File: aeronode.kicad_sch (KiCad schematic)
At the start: 8 parts

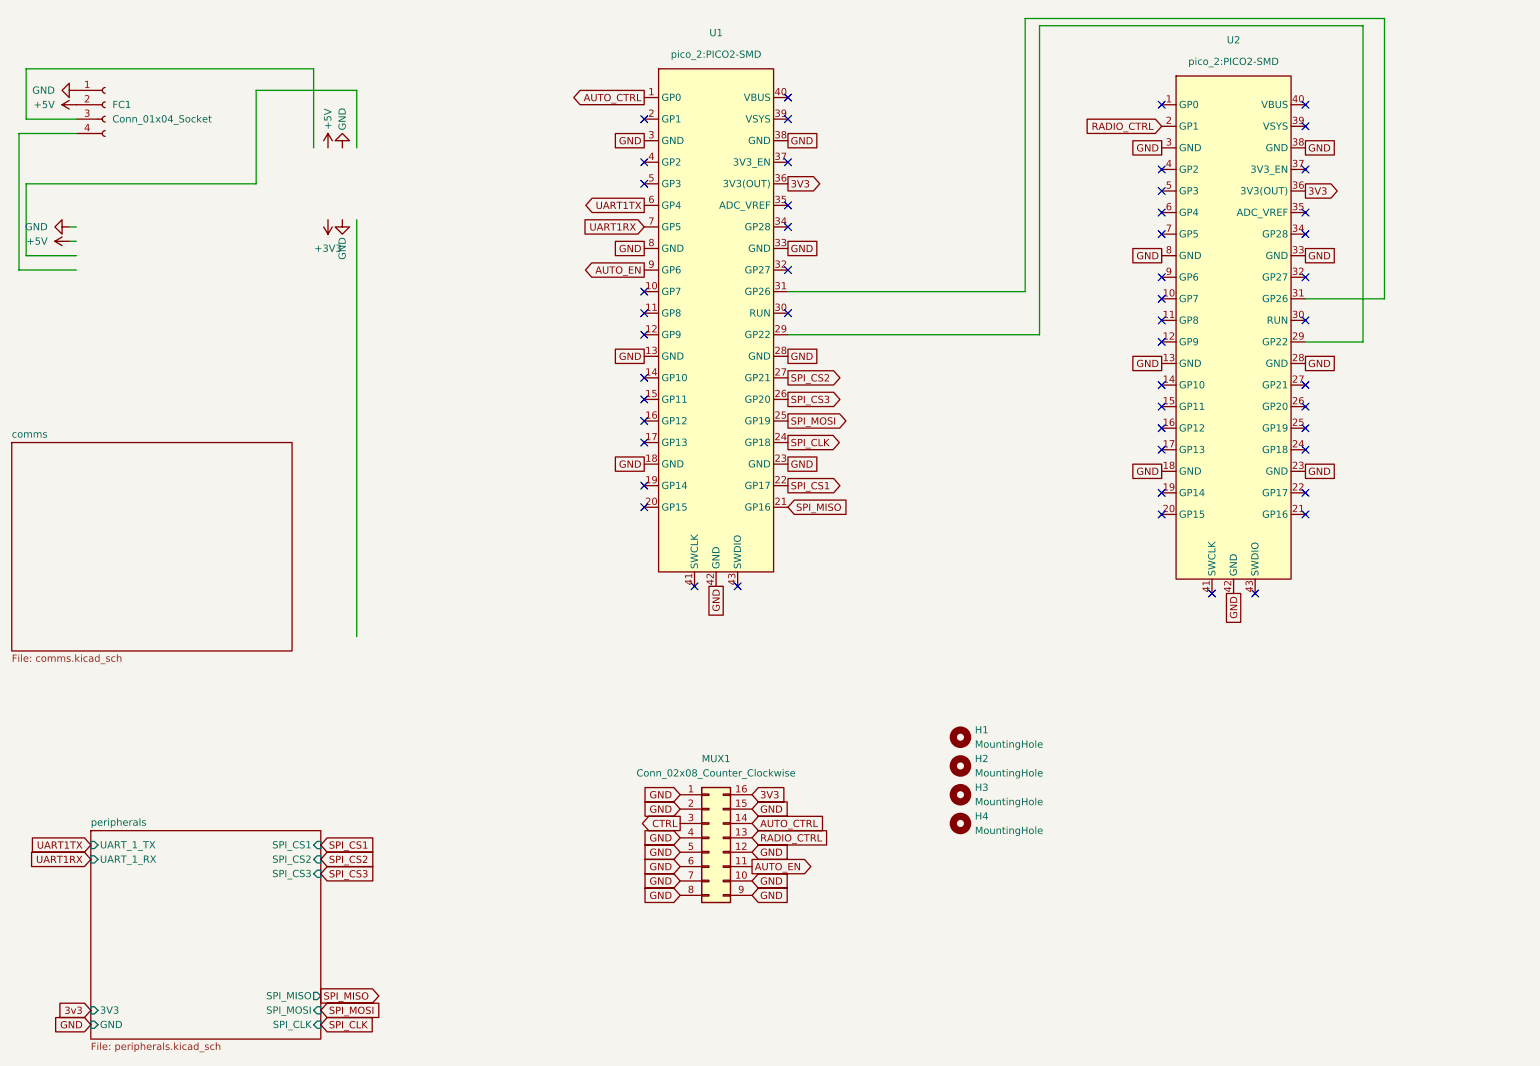
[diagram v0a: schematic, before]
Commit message: v0.1
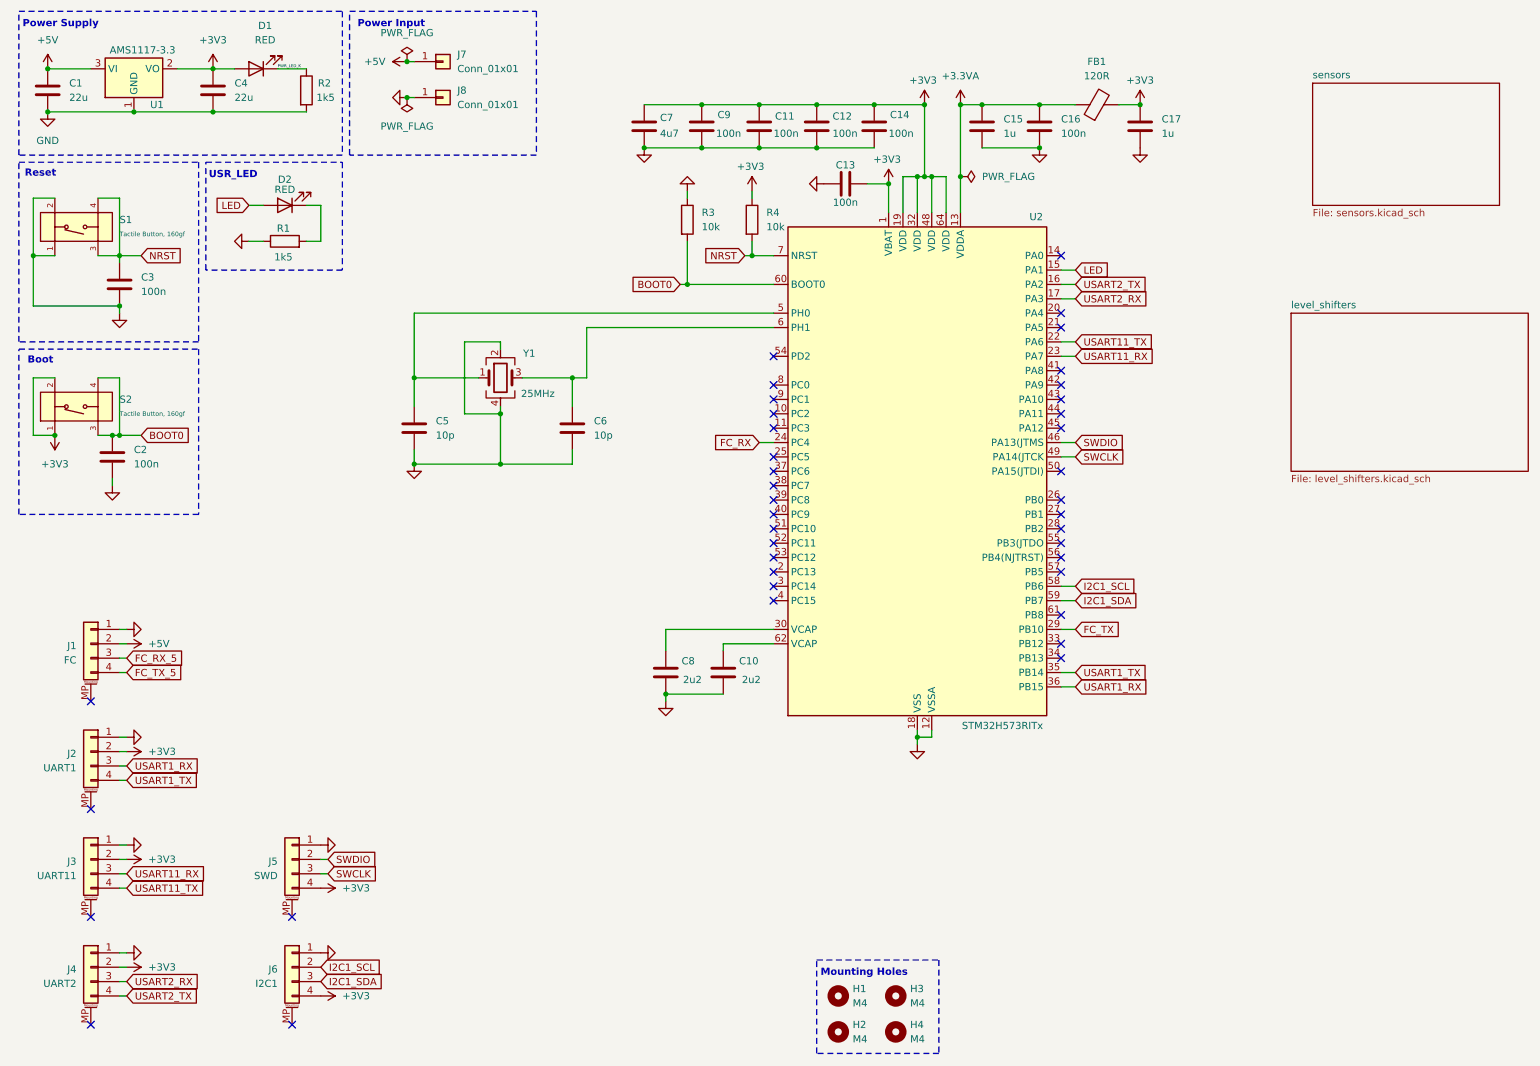
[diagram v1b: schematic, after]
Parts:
- removed FC1: Conn_01x04_Socket, Connector_PinSocket_2.54mm:PinSocket_1x04_P2.54mm_Vertical, symbol Connector:Conn_01x04_Socket
- removed MUX1: Conn_02x08_Counter_Clockwise, Connector_PinHeader_2.54mm:PinHeader_2x8_2.54mm_7.62mm, symbol Connector_Generic:Conn_02x08_Counter_Clockwise
- removed U1, U2: ~, pico_2:PICO2-SMD, symbol pico_2:PICO2-SMD
- added C1, C4: 22u, Capacitor_SMD:C_0805_2012Metric, symbol Device:C
- added C10, C8: 2u2, Capacitor_SMD:C_0402_1005Metric, symbol Device:C
- added C11, C12, C13, C14, C16, C2, C3, C9: 100n, Capacitor_SMD:C_0402_1005Metric, symbol Device:C
- added C15, C17: 1u, Capacitor_SMD:C_0402_1005Metric, symbol Device:C
- added C5, C6: 10p, Capacitor_SMD:C_0402_1005Metric, symbol Device:C
- added C7: 4u7, Capacitor_SMD:C_0603_1608Metric, symbol Device:C
- added D1, D2: RED, LED_SMD:LED_0603_1608Metric, symbol Device:LED
- added FB1: 120R, Inductor_SMD:L_0603_1608Metric, symbol Device:FerriteBead
- added J1: FC, Connector_JST:JST_GH_SM04B-GHS-TB_1x04-1MP_P1.25mm_Horizontal, symbol Connector_Generic_MountingPin:Conn_01x04_MountingPin
- added J2: UART1, Connector_JST:JST_GH_SM04B-GHS-TB_1x04-1MP_P1.25mm_Horizontal, symbol Connector_Generic_MountingPin:Conn_01x04_MountingPin
- added J3: UART11, Connector_JST:JST_GH_SM04B-GHS-TB_1x04-1MP_P1.25mm_Horizontal, symbol Connector_Generic_MountingPin:Conn_01x04_MountingPin
- added J4: UART2, Connector_JST:JST_GH_SM04B-GHS-TB_1x04-1MP_P1.25mm_Horizontal, symbol Connector_Generic_MountingPin:Conn_01x04_MountingPin
- added J5: SWD, Connector_JST:JST_GH_SM04B-GHS-TB_1x04-1MP_P1.25mm_Horizontal, symbol Connector_Generic_MountingPin:Conn_01x04_MountingPin
- added J6: I2C1, Connector_JST:JST_GH_SM04B-GHS-TB_1x04-1MP_P1.25mm_Horizontal, symbol Connector_Generic_MountingPin:Conn_01x04_MountingPin
- added J7, J8: Conn_01x01, Connector_Wire:SolderWirePad_1x01_SMD_2x4mm, symbol Connector_Generic:Conn_01x01
- added R1, R2: 1k5, Resistor_SMD:R_0402_1005Metric, symbol Device:R
- added R3, R4: 10k, Resistor_SMD:R_0402_1005Metric, symbol Device:R
- added S1, S2: Tactile Button, 160gf, PCM_JLCPCB:SW-SMD_4P-L5.1-W5.1-P3.70-LS6.5-TL-2, symbol PCM_JLCPCB-Connectors_Buttons:Tactile Button, 160gf, 12V, 50mA, 5.1mm
- added U1: AMS1117-3.3, Package_TO_SOT_SMD:SOT-223-3_TabPin2, symbol Regulator_Linear:AMS1117-3.3
- added U2: STM32H573RITx, Package_QFP:LQFP-64_10x10mm_P0.5mm, symbol MCU_ST_STM32H5:STM32H573RITx
- added Y1: 25MHz, Crystal:Crystal_SMD_3225-4Pin_3.2x2.5mm, symbol Device:Crystal_GND24
- H1, H2, H3, H4: value MountingHole -> M4; footprint (none) -> MountingHole:MountingHole_4.3mm_M4
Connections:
- net +3V3: now also C11.1, C12.1, C13.2, C14.1, C17.2, C4.1, C7.1, C9.1, D1.2 (A), FB1.2, J2.2 (Pin_2), J3.2 (Pin_2), J4.2 (Pin_2), J5.4 (Pin_4), J6.4 (Pin_4), R4.1, S2.1 (A), S2.2 (B), U1.2 (VO), U2.1 (VBAT), U2.19 (VDD), U2.32 (VDD), U2.48 (VDD), U2.64 (VDD)
- net +5V: now also C1.1, J1.2 (Pin_2), J7.1 (Pin_1), U1.3 (VI)
- net GND: now also C1.2, C10.2, C11.2, C12.2, C13.1, C14.2, C15.1, C16.1, C17.1, C2.2, C3.2, C4.2, C5.2, C6.2, C7.2, C8.2, C9.2, J1.1 (Pin_1), J2.1 (Pin_1), J3.1 (Pin_1), J4.1 (Pin_1), J5.1 (Pin_1), J6.1 (Pin_1), J8.1 (Pin_1), R1.1, R2.2, R3.1, S1.1 (A), S1.2 (B), U1.1 (GND), U2.12 (VSSA), U2.18 (VSS), U2.31 (VSS), U2.47 (VSS), U2.63 (VSS), Y1.2, Y1.4
- new net: C8.1, U2.30 (VCAP)
- new net: C5.1, U2.5 (PH0), Y1.1
- new net: C6.1, U2.6 (PH1), Y1.3
- new net: C10.1, U2.62 (VCAP)
- new net: D2.1 (K), R1.2
- new net +3.3VA: C15.2, C16.2, FB1.1, U2.13 (VDDA)
- new net BOOT0: C2.1, R3.2, S2.3 (C), S2.4 (D), U2.60 (BOOT0)
- new net FC_RX: U2.24 (PC4)
- new net FC_RX_5: J1.3 (Pin_3)
- new net FC_TX: U2.29 (PB10)
- new net FC_TX_5: J1.4 (Pin_4)
- new net I2C1_SCL: J6.2 (Pin_2), U2.58 (PB6)
- new net I2C1_SDA: J6.3 (Pin_3), U2.59 (PB7)
- new net LED: D2.2 (A), U2.15 (PA1)
- new net NRST: C3.1, R4.2, S1.3 (C), S1.4 (D), U2.7 (NRST)
- new net PWR_LED_K: D1.1 (K), R2.1
- new net SWCLK: J5.3 (Pin_3), U2.49 (PA14(JTCK)
- new net SWDIO: J5.2 (Pin_2), U2.46 (PA13(JTMS)
- new net USART11_RX: J3.3 (Pin_3), U2.23 (PA7)
- new net USART11_TX: J3.4 (Pin_4), U2.22 (PA6)
- new net USART1_RX: J2.3 (Pin_3), U2.36 (PB15)
- new net USART1_TX: J2.4 (Pin_4), U2.35 (PB14)
- new net USART2_RX: J4.3 (Pin_3), U2.17 (PA3)
- new net USART2_TX: J4.4 (Pin_4), U2.16 (PA2)
- no-connect marks 51 -> 40
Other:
- removed sheet comms
- removed sheet peripherals
- added sheet level_shifters (level_shifters.kicad_sch)
- added sheet sensors (sensors.kicad_sch)
- note added: "Boot"
- note added: "Mounting Holes"
- note added: "Power Input"
- note added: "Power Supply"
- note added: "Reset"
- note added: "USR_LED"
- company: Moonlit Garage, Inc -> Moonlit Garage, Inc.
- title: aeronode -> AeroNode
